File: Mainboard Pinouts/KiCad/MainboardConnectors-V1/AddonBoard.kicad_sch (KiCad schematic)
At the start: 9 parts, among them M1 Fan_External(40mm), M2 Fan_Recirculating, Q2 Q_NMOS

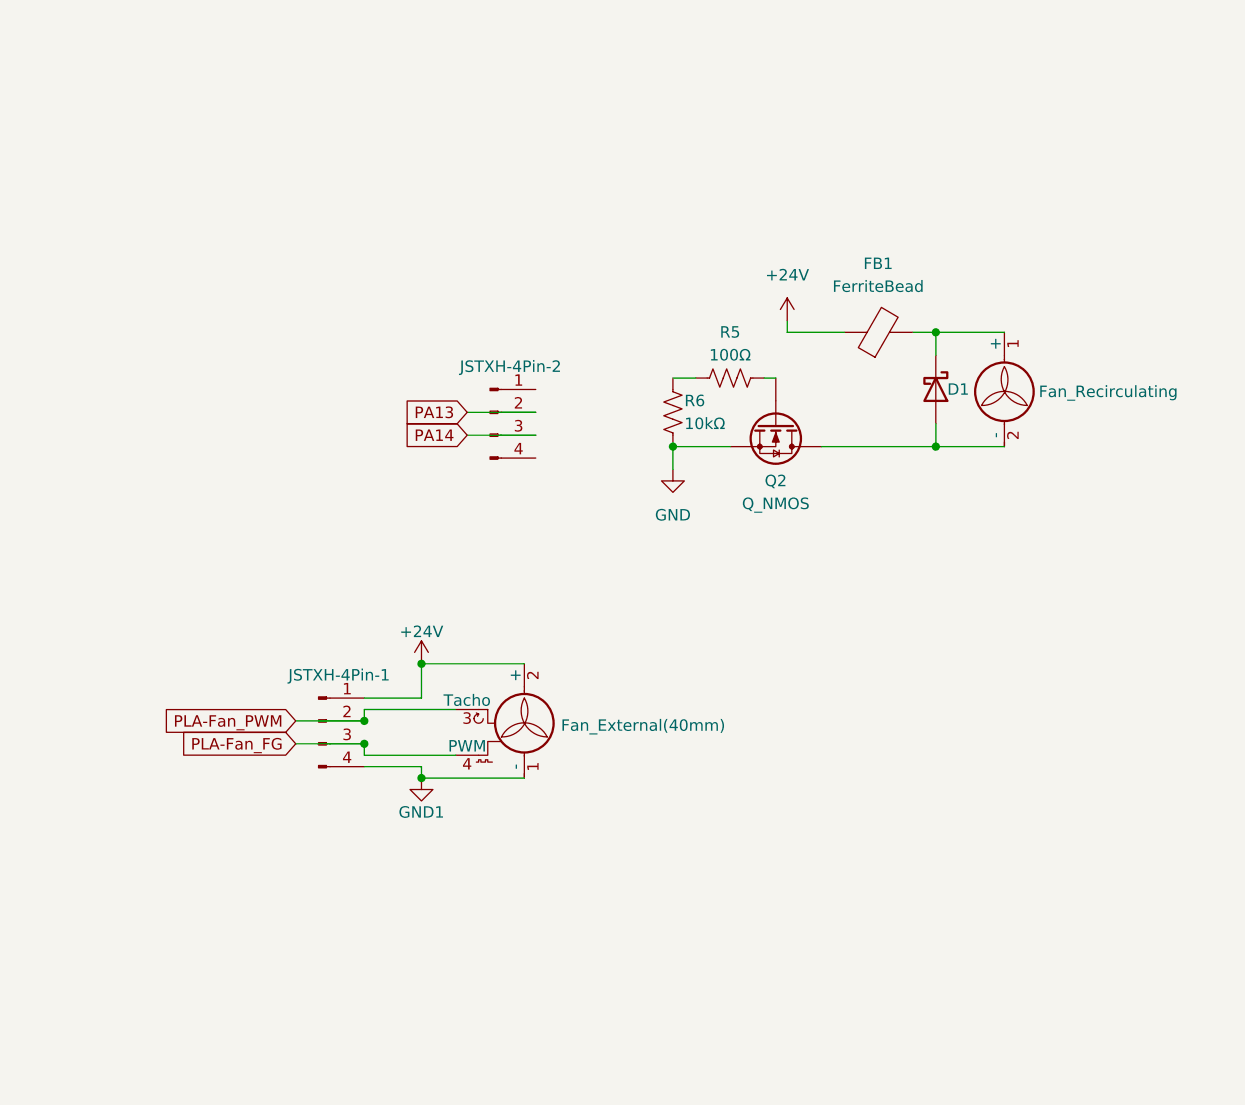
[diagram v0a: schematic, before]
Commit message: Finished V1 build of addon board
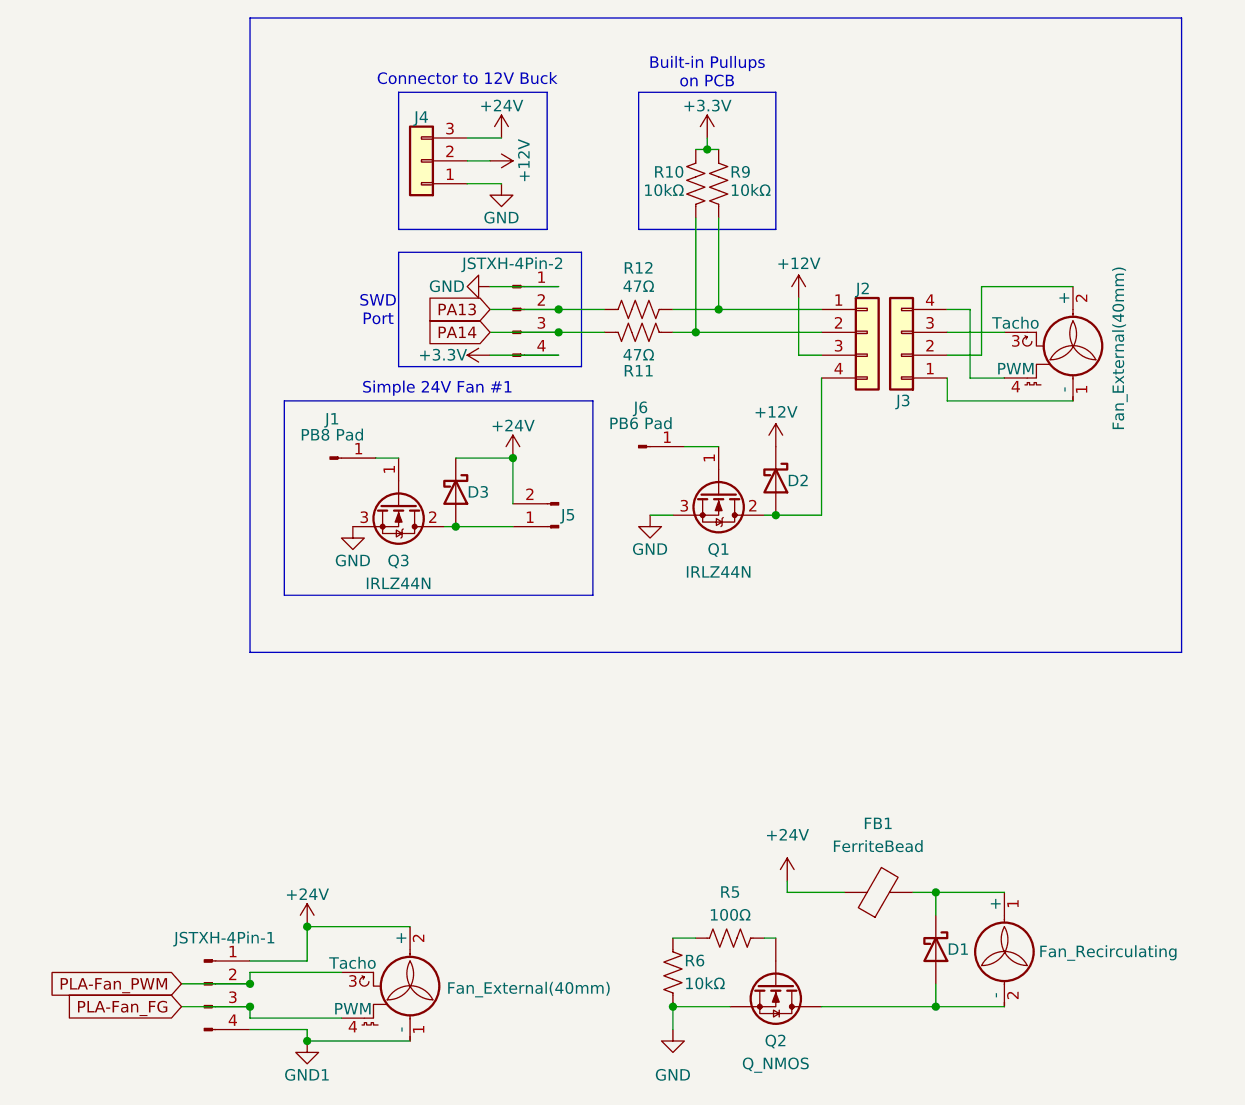
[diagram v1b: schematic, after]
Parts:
- added D2, D3: D_Schottky, symbol Device:D_Schottky
- added J1: PB8 Pad, symbol Connector:Conn_01x01_Pin
- added J2, J3: Conn_01x04, symbol Connector_Generic:Conn_01x04
- added J4: Conn_01x03, symbol Connector_Generic:Conn_01x03
- added J5: Conn_01x02_Pin, symbol Connector:Conn_01x02_Pin
- added J6: PB6 Pad, symbol Connector:Conn_01x01_Pin
- added M3: Fan_External(40mm), symbol Motor:Fan_4pin
- added Q1, Q3: IRLZ44N, Package_TO_SOT_THT:TO-220-3_Vertical, symbol Transistor_FET:IRLZ44N
- added R10, R9: 10kΩ, symbol Device:R_US
- added R11, R12: 47Ω, symbol Device:R_US
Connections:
- net +24V: now also D3.1 (K), J4.3 (Pin_3), J5.2 (Pin_2)
- net GND: now also JSTXH-4Pin-2.1 (Pin_1), J4.1 (Pin_1), Q1.3 (S), Q3.3 (S)
- net PA13: now also R12.1
- net PA14: now also R11.1
- net +3.3V: now reaches JSTXH-4Pin-2.4 (Pin_4)
- net +3.3V: now also R10.1, R9.1
- new net: J2.2 (Pin_2), R10.2, R11.2
- new net: J1.1 (Pin_1), Q3.1 (G)
- new net: D3.2 (A), J5.1 (Pin_1), Q3.2 (D)
- new net: J2.1 (Pin_1), R12.2, R9.2
- new net: D2.2 (A), J2.4 (Pin_4), Q1.2 (D)
- new net: J3.1 (Pin_1), M3.1 (-)
- new net: J3.2 (Pin_2), M3.2 (+)
- new net: J3.3 (Pin_3), M3.3 (Tacho)
- new net: J3.4 (Pin_4), M3.4 (PWM)
- new net: J6.1 (Pin_1), Q1.1 (G)
- new net +12V: D2.1 (K), J2.3 (Pin_3), J4.2 (Pin_2)
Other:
- note added: "Built-in Pullups on PCB"
- note added: "Connector to 12V Buck"
- note added: "SWD Port"
- note added: "Simple 24V Fan #1"
- moved on the sheet: D1, FB1, JSTXH-4Pin-1, JSTXH-4Pin-2, Q2, R5, R6
